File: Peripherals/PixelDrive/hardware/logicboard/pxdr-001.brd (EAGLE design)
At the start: 92 x 58 mm, 12 parts

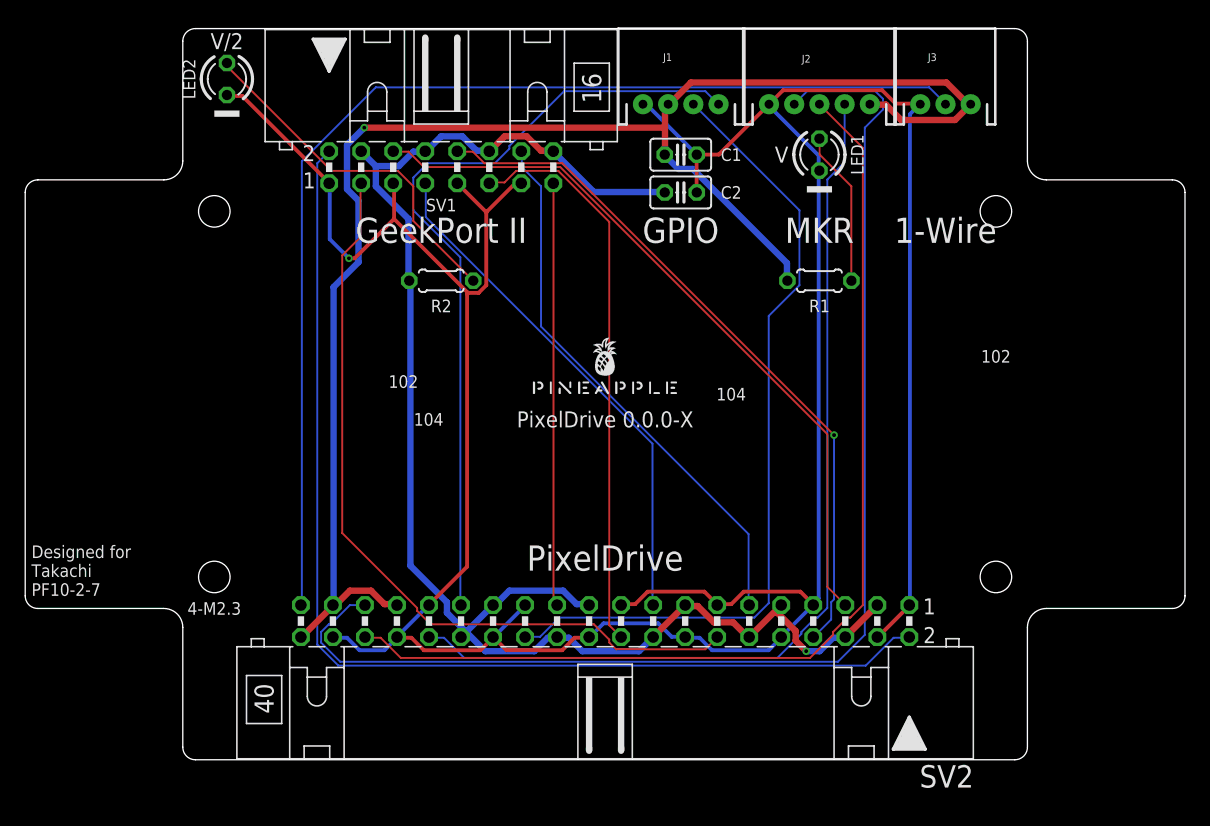
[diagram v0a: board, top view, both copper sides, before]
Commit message: Third shot.
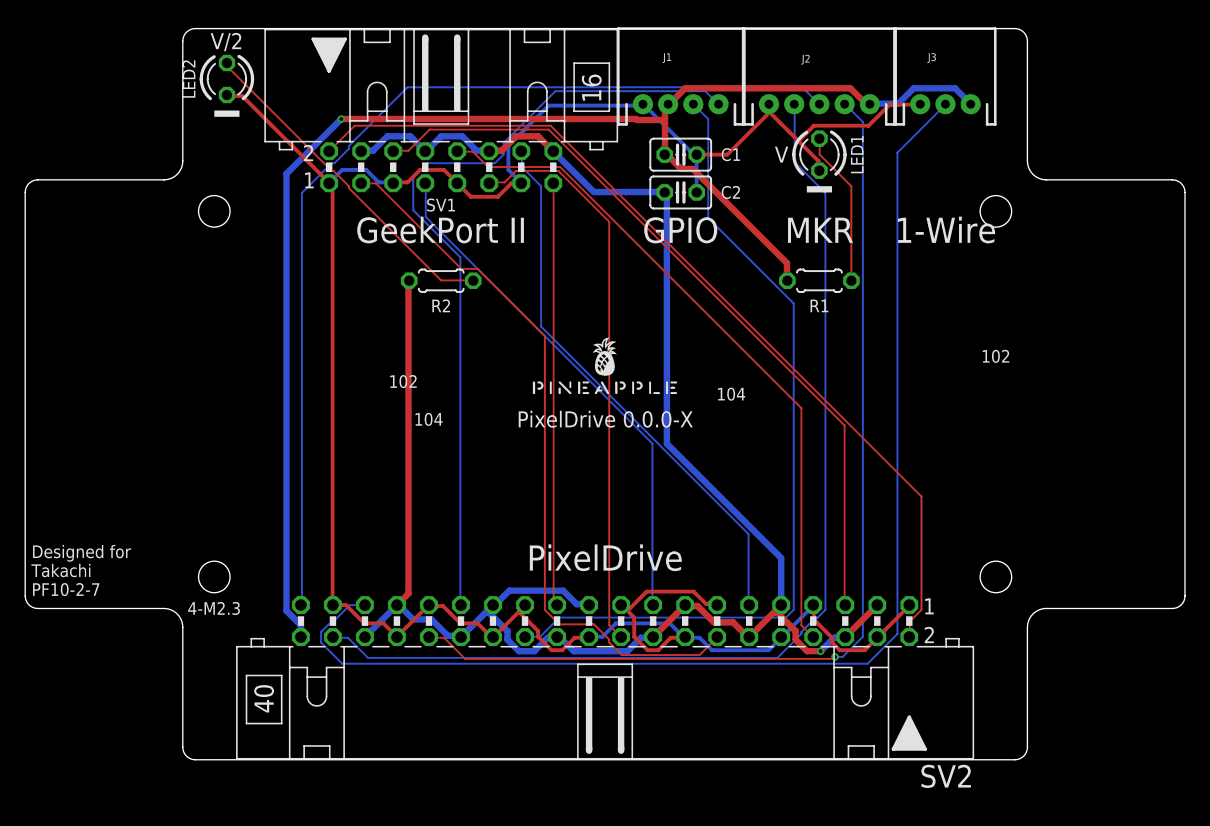
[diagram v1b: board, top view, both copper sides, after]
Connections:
- net DIGITAL7 renamed NP11
- removed net THS: J3.2, SV2.39
- new net NP12: J3.2, SV2.35
- net GND: now also SV2.37; no longer SV2.38
- net SCL: now also SV2.39; no longer SV2.36
- net SDA: now also SV2.38; no longer SV2.35
- net VCC: no longer SV2.33, SV2.37
- net VCC/2: now also SV2.33, SV2.36
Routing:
- net NP12: track 0.00 -> 96.2 mm
- net THS: track 89.3 -> 0.00 mm
- net GND: track 256.8 -> 188.7 mm, vias 1 -> 0
- net VCC/2: track 123.2 -> 154.7 mm
- net SDA: track 100.7 -> 82.6 mm
- net NP1: track 88.1 -> 71.6 mm
- net VCC: track 126.5 -> 113.9 mm
- net NP5: track 62.6 -> 57.2 mm
- net SCL: track 83.2 -> 77.9 mm
- net NP11: track 74.5 -> 78.7 mm, vias 0 -> 1
- net NP2: track 57.9 -> 60.5 mm
- net NP3: track 55.9 -> 54.3 mm, vias 1 -> 0
- net VCC2LED: track 28.4 -> 26.9 mm
- net NP9: track 64.5 -> 65.6 mm
